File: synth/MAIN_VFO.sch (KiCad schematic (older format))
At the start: 39 parts

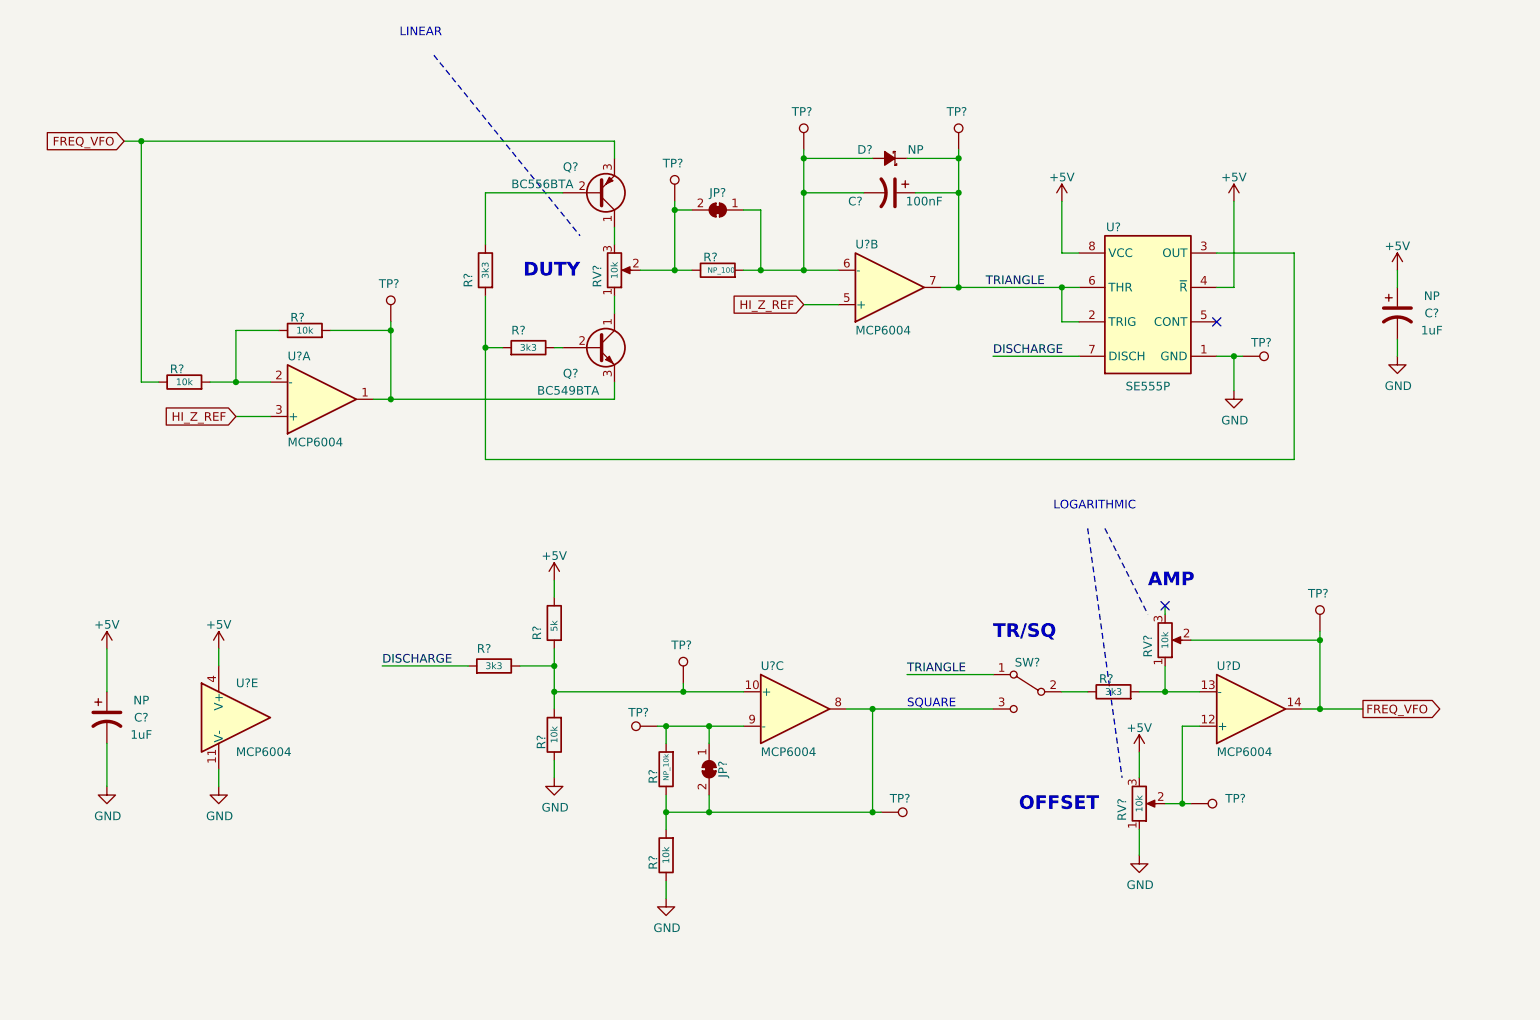
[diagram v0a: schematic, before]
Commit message: automated commit
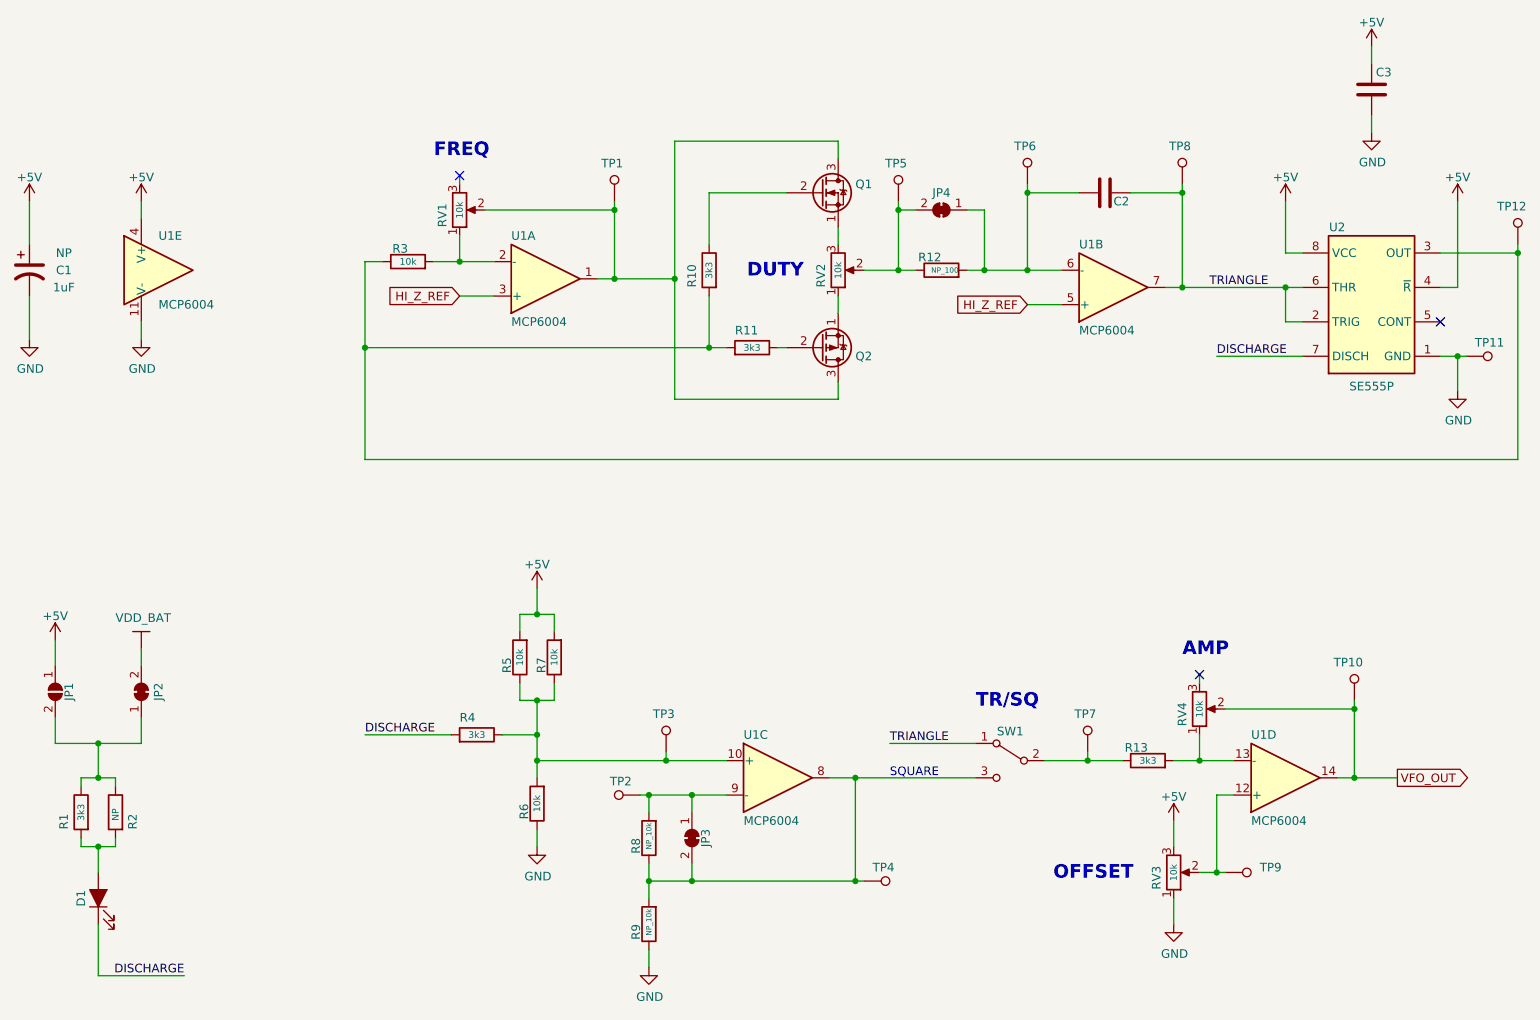
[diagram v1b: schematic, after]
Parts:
- removed C?: 100nF, symbol Device:CP1
- removed C? (x2): 1uF, symbol Device:CP1
- removed D?: D_Schottky_Small_ALT, symbol Device:D_Schottky_Small_ALT
- removed JP? (x2): SolderJumper_2_Bridged, symbol Jumper:SolderJumper_2_Bridged
- removed Q?: BC549BTA, symbol Device:Q_NPN_CBE
- removed Q?: BC556BTA, symbol Device:Q_PNP_CBE
- removed R?: NP_100, symbol Device:R
- removed R? (x4): 10k, symbol Device:R
- removed R? (x4): 3k3, symbol Device:R
- removed R?: 5k, symbol Device:R
- removed R?: NP_10k, symbol Device:R
- removed RV? (x3): 10k, symbol Device:R_POT
- removed SW?: SW_SPDT, symbol Switch:SW_SPDT
- removed TP? (x10): PTH_1_mm, TestPoint:TestPoint_THTPad_D2.0mm_Drill1.0mm, symbol custom:PTH_1_mm
- removed U?: SE555P, symbol custom:SE555P
- removed U? (x5): MCP6004, Package_DIP:DIP-14_W7.62mm_LongPads, symbol custom:MCP6004
- added C1: 1uF, symbol Device:CP1
- added C2, C3: C, symbol Device:C
- added D1: LED_ALT, symbol Device:LED_ALT
- added JP1: SolderJumper_2_Open, symbol Jumper:SolderJumper_2_Open
- added JP2, JP3, JP4: SolderJumper_2_Bridged, symbol Jumper:SolderJumper_2_Bridged
- added Q1: Q_NMOS_SGD, symbol Device:Q_NMOS_SGD
- added Q2: Q_PMOS_SGD, symbol Device:Q_PMOS_SGD
- added R1, R10, R11, R13, R4: 3k3, symbol Device:R
- added R12: NP_100, symbol Device:R
- added R2: NP, symbol Device:R
- added R3, R5, R6, R7: 10k, symbol Device:R
- added R8, R9: NP_10k, symbol Device:R
- added RV1, RV2, RV3, RV4: 10k, symbol Device:R_POT
- added SW1: SW_SPDT, symbol Switch:SW_SPDT
- added TP1, TP10, TP11, TP12, TP2, TP3, TP4, TP5, TP6, TP7, TP8, TP9: PTH_1_mm, TestPoint:TestPoint_THTPad_D2.0mm_Drill1.0mm, symbol custom:PTH_1_mm
- added U1: MCP6004, Package_DIP:DIP-14_W7.62mm_LongPads, symbol custom:MCP6004
- added U2: SE555P, symbol custom:SE555P
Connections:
- net +5V: now also C1.1, C3.1, JP1.1 (A), R5.2, R7.2, RV3.3, U1.4 (V+), U2.4 (~R), U2.8 (VCC)
- net DISCHARGE: now also D1.1 (K), R4.2, U2.7 (DISCH)
- net GND: now also C1.2, C3.2, R6.1, R9.1, RV3.1, TP11.1, U1.11 (V-), U2.1 (GND)
- net HI_Z_REF: now also U1.3 (+), U1.5 (+)
- net TRIANGLE: now also C2.1, SW1.1 (A), TP8.1, U1.7, U2.2 (TRIG), U2.6 (THR)
- new net: Q1.2 (G), R10.1
- new net: R10.2, R11.2, R3.1, TP12.1, U2.3 (OUT)
- new net: Q2.2 (G), R11.1
- new net: C2.2, JP4.1 (A), R12.2, TP6.1, U1.6 (-)
- new net: JP4.2 (B), R12.1, RV2.2, TP5.1
- new net: R4.1, R5.1, R6.2, R7.1, TP3.1, U1.10 (+)
- new net: JP3.1 (A), R8.2, TP2.1, U1.9 (-)
- new net: JP3.2 (B), R8.1, R9.2, SW1.3 (C), TP4.1, U1.8
- new net: RV3.2, TP9.1, U1.12 (+)
- new net: Q1.3 (D), Q2.3 (D), RV1.2, TP1.1, U1.1
- new net: R13.1, SW1.2 (B), TP7.1
- new net: R13.2, RV4.1, U1.13 (-)
- new net: Q2.1 (S), RV2.1
- new net: Q1.1 (S), RV2.3
- new net: R3.2, RV1.1, U1.2 (-)
- new net: JP1.2 (B), JP2.1 (A), R1.1, R2.1
- new net: D1.2 (A), R1.2, R2.2
- new net VDD_BAT: JP2.2 (B)
- new net VFO_OUT: RV4.2, TP10.1, U1.14
- no-connect marks 2 -> 3
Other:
- note added: "FREQ"
- note removed: "LINEAR"
- note removed: "LOGARITHMIC"
